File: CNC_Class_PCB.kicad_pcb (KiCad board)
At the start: 2 copper layers, 103.5 x 109.7 mm, 16 parts, among them Q2 2N3904, U1 ICM7555xB

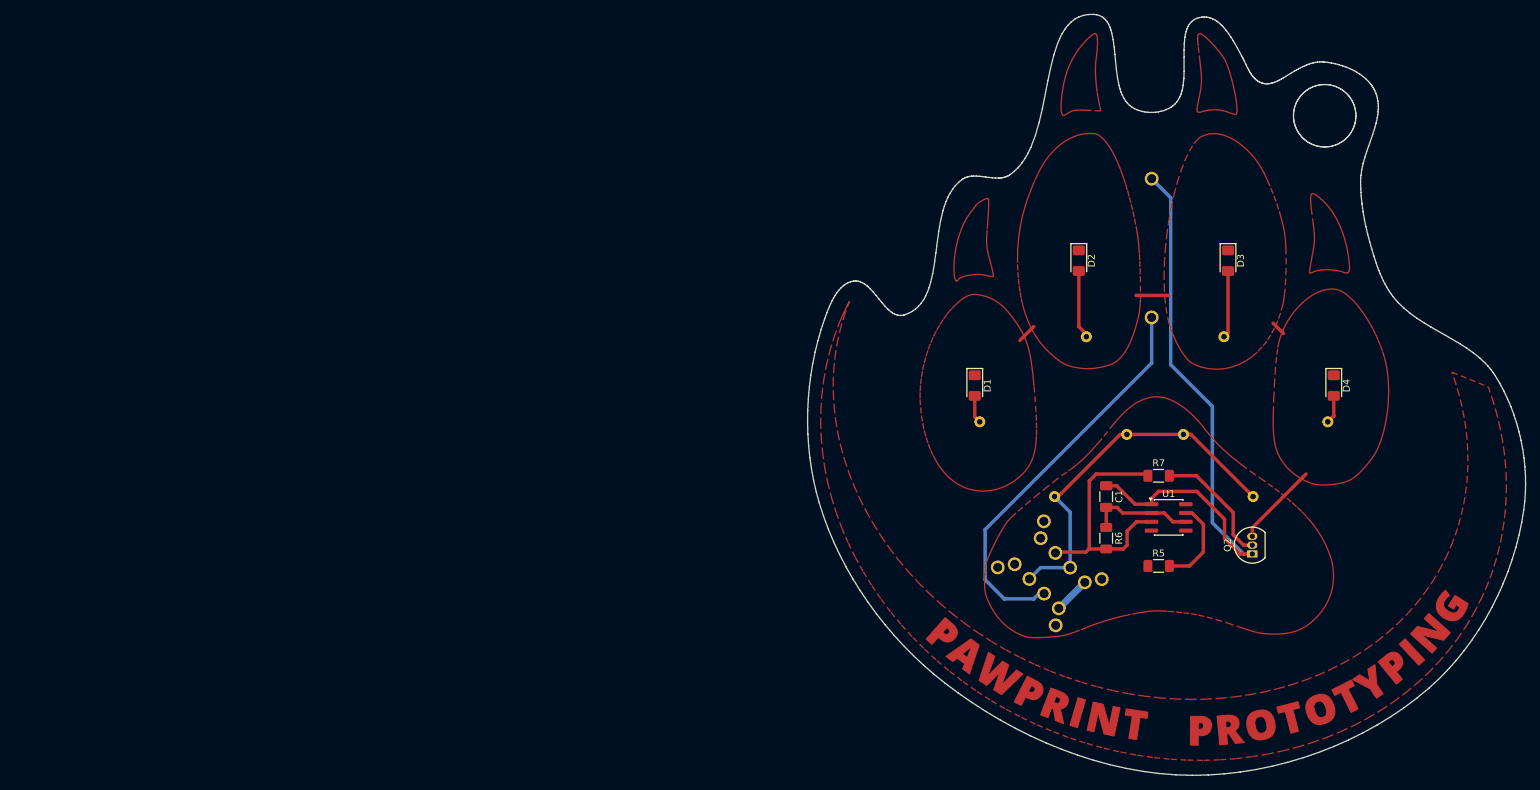
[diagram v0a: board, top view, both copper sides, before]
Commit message: smol
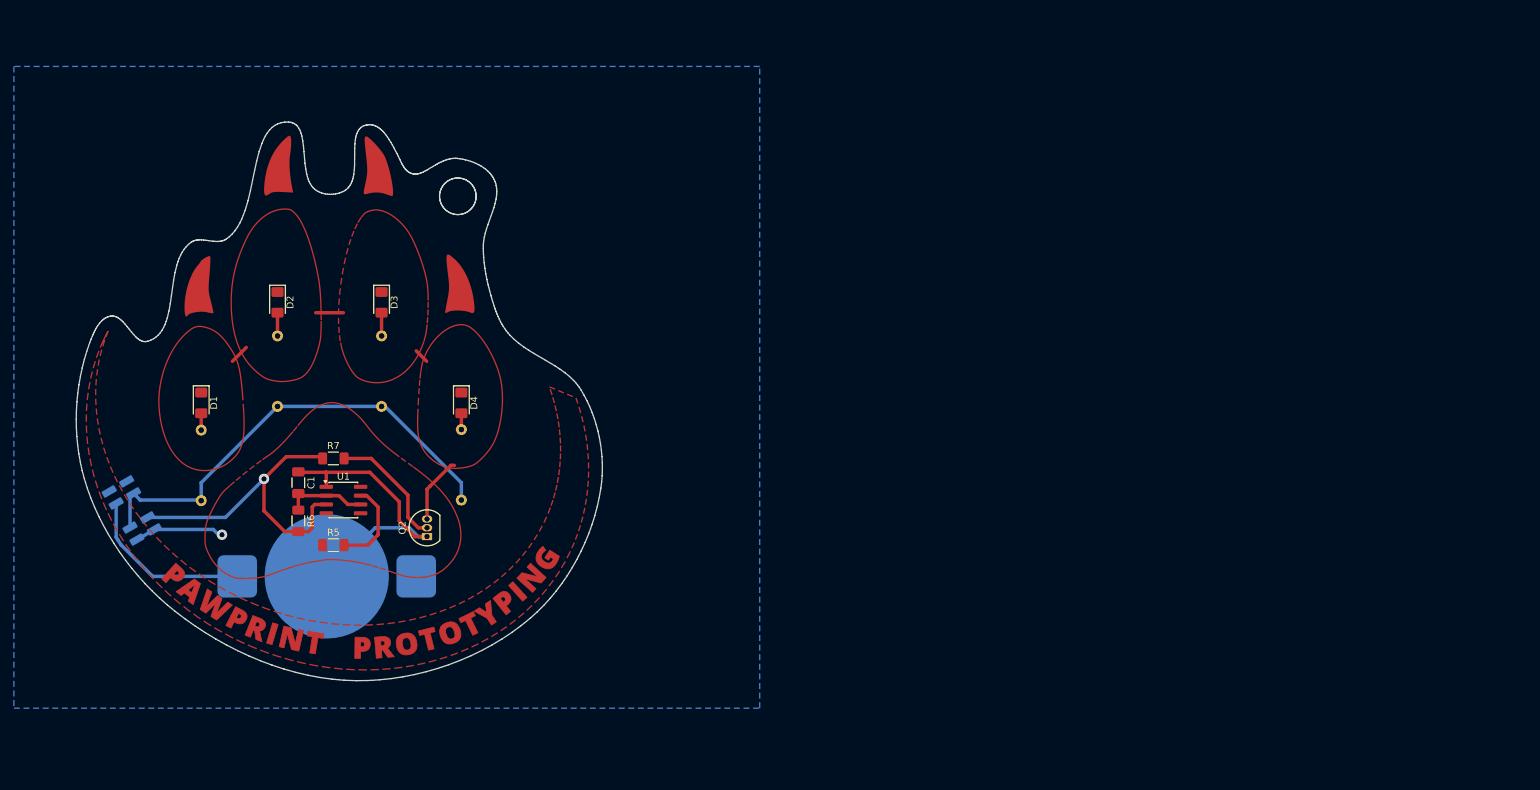
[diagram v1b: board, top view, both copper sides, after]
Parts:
- removed S1: ~, My_Library:OS203013MT6QN1
- added SW1: ~, My_Library:SLW-133538-2A-SMT-TR, B.Cu at (50.0, 106.0)
- BT1: footprint My_Library:BH-25C-1 -> My_Library:BAT-HLD-003-SMT
- R1, R2, R3, R4: footprint Resistor_THT:R_Axial_DIN0207_L6.3mm_D2.5mm_P15.24mm_Horizontal -> Resistor_THT:R_Axial_DIN0207_L6.3mm_D2.5mm_P10.16mm_Horizontal
- moved BT1 129.2 mm to (78.1, 115.5), turned to 180 degrees
- moved D4 125.8 mm to (97.5, 90.5)
- moved R1 123.0 mm to (60.0, 104.6), turned to 90 degrees
- moved R2 122.5 mm to (71.0, 91.0), turned to 90 degrees
- moved D3 122.1 mm to (86.0, 76.0)
- moved R5 119.0 mm to (79.0, 111.0)
- moved Q2 119.0 mm to (92.5, 109.8)
- moved R7 119.0 mm to (79.0, 98.5)
- moved U1 119.0 mm to (80.5, 104.5)
- moved R6 116.5 mm to (74.0, 107.5)
- moved C1 116.5 mm to (74.0, 102.0)
- moved D2 115.7 mm to (71.0, 76.0)
- moved R3 115.7 mm to (86.0, 91.0), turned to 90 degrees
- moved R4 114.1 mm to (97.5, 104.5), turned to 90 degrees
- moved D1 111.5 mm to (60.0, 90.5)
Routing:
- net GND: track 89.6 -> 44.0 mm
- net +BATT: track 57.7 -> 24.8 mm
- net Vdrive: track 53.9 -> 67.0 mm
- net Net-(U1-Q): track 35.7 -> 47.2 mm, vias 0 -> 1
- net VCC: track 5.30 -> 13.0 mm, vias 0 -> 1
- net Net-(D2-A): track 9.92 -> 2.46 mm
- net Net-(D3-A): track 9.83 -> 2.46 mm
- net Net-(D1-K): track 21.9 -> 18.6 mm
- net Net-(U1-THR): track 15.2 -> 12.0 mm
- net Net-(D1-A): track 4.04 -> 2.01 mm
- net Net-(D4-A): track 4.09 -> 2.46 mm
- added copper zone on B.Cu, net (none)
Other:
- board size 103.5 x 109.7 mm -> 75.8 x 80.5 mm
